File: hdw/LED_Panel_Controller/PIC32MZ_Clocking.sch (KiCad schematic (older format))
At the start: 16 parts

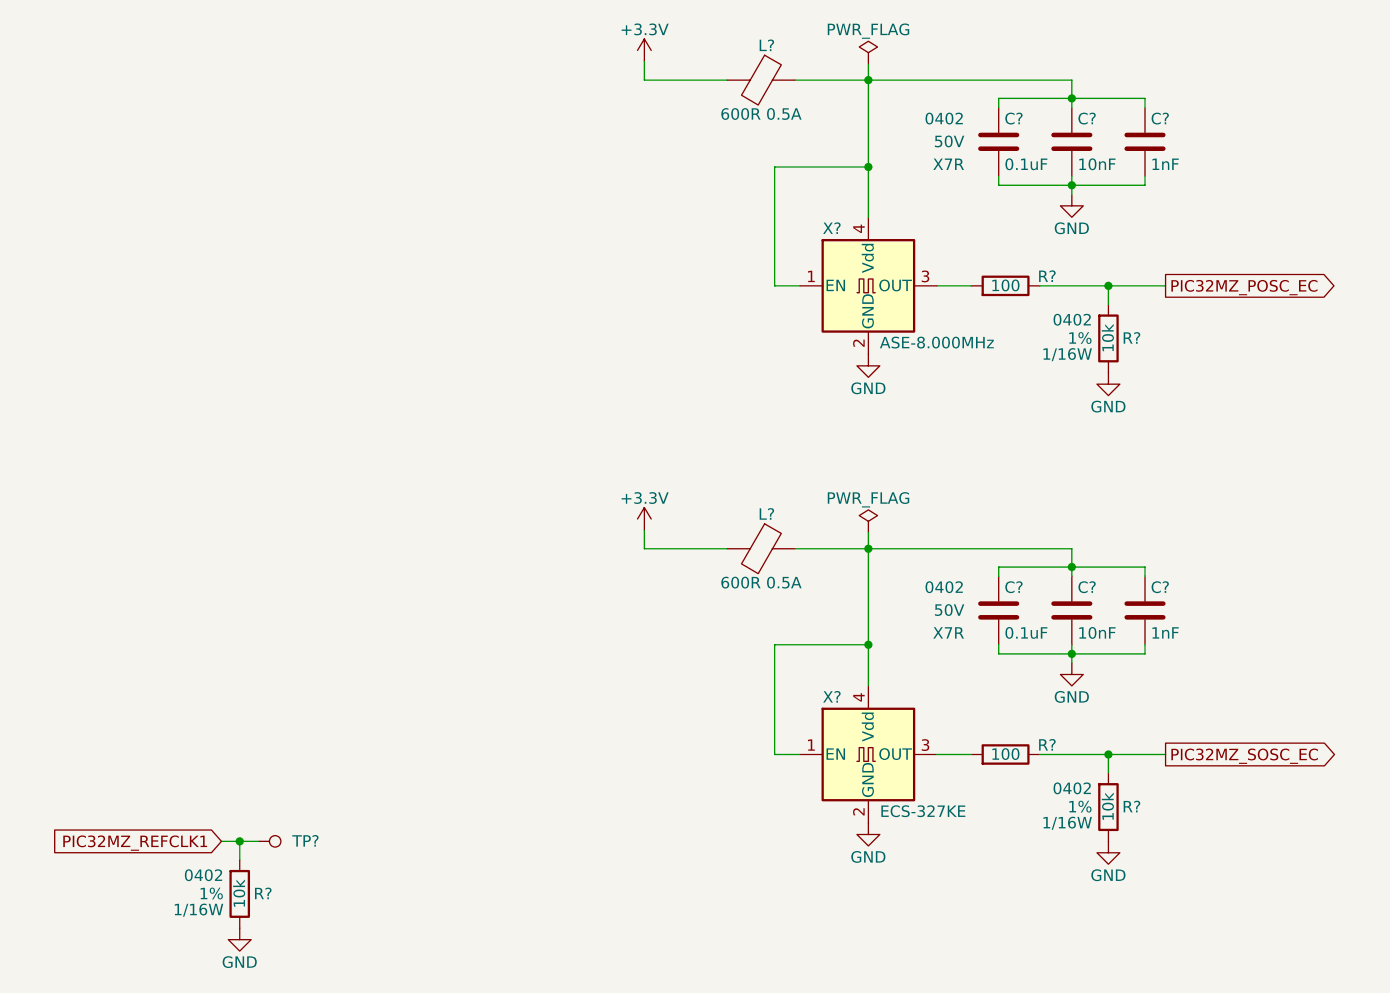
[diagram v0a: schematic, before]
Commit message: lots of schematic progress
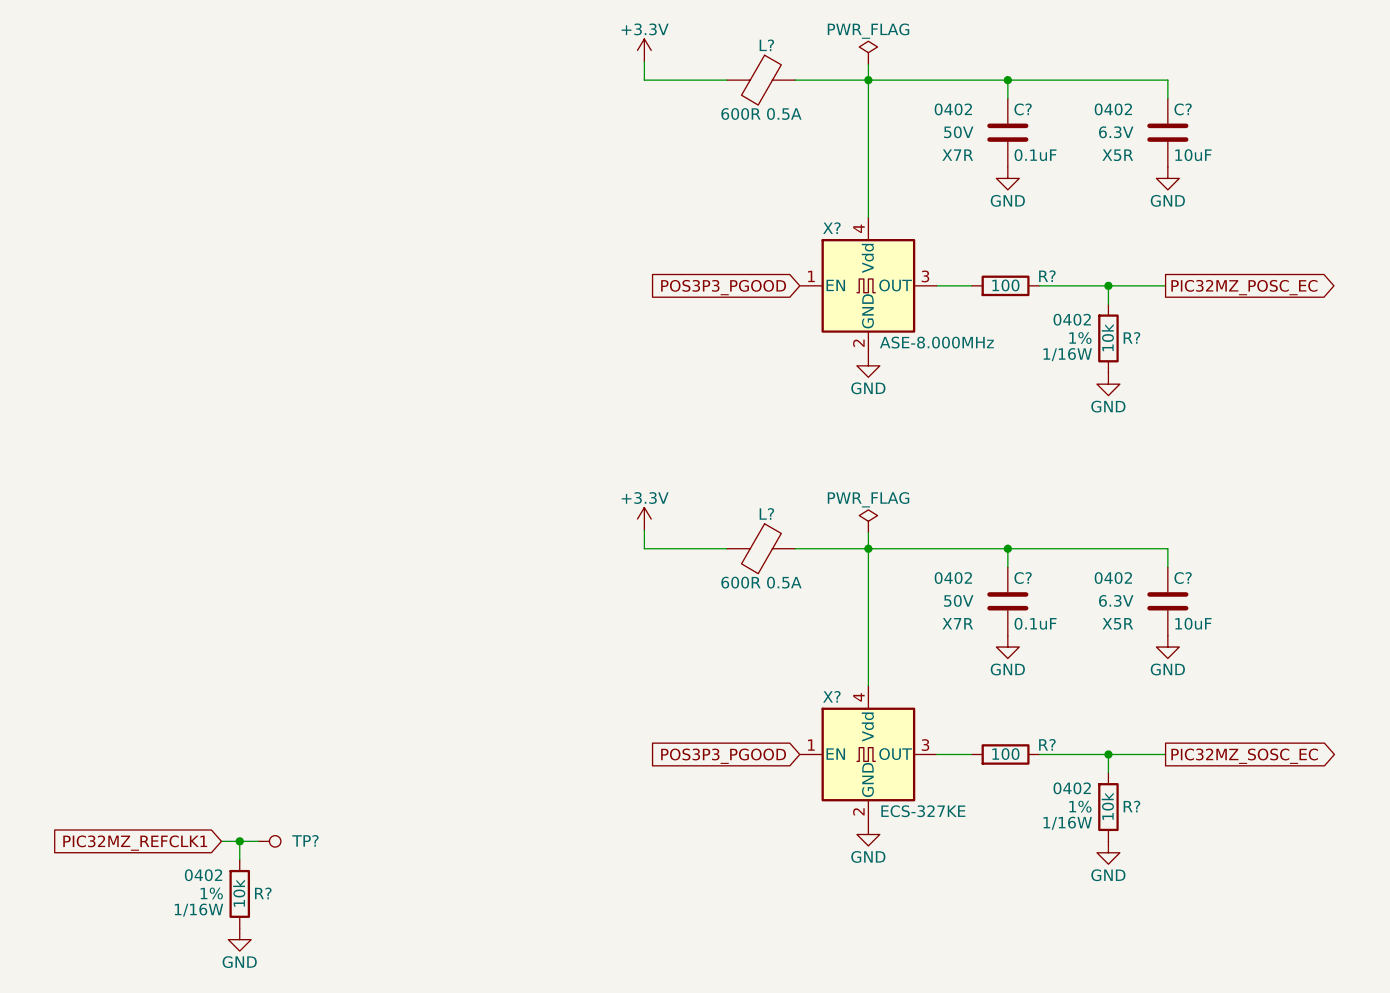
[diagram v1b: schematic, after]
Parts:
- removed C? (x2): 0.1uF, Capacitors_SMD:C_0402, symbol Custom_Library:C_Custom
- removed C? (x2): 1nF, Capacitors_SMD:C_0402, symbol Custom_Library:C_Custom
- removed C? (x2): 10nF, Capacitors_SMD:C_0402, symbol Custom_Library:C_Custom
- added C? (x2): 0.1uF, Capacitors_SMD:C_0402, symbol Custom_Library:C_Custom
- added C? (x2): 10uF, Capacitors_SMD:C_0402, symbol Custom_Library:C_Custom
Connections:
- net GND: now also C?.2, C?.2, C?.2, C?.2
- net at L?.1, X?.4 (Vdd): now also C?.1, C?.1; no longer X?.1 (EN) (x2)
- new net POS3P3_PGOOD: X?.1 (EN), X?.1 (EN)
